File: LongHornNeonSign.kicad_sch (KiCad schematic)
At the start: 61 parts, among them J1 Screw_Terminal_01x02, J2 Screw_Terminal_01x02, J3 Screw_Terminal_01x02, J4 Screw_Terminal_01x02, Q1 AO3400A, Q2 AO3400A, Q3 AO3400A, Q4 AO3400A, SW1 SW_Push, SW2 SW_Push, SW3 SW_Push, U1 LM2596S-5

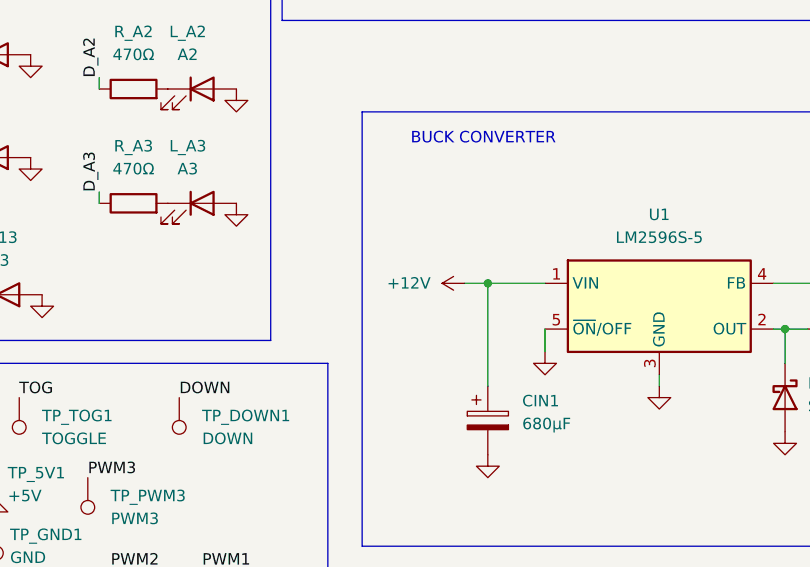
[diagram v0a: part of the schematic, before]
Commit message: May 12 2026 run it back
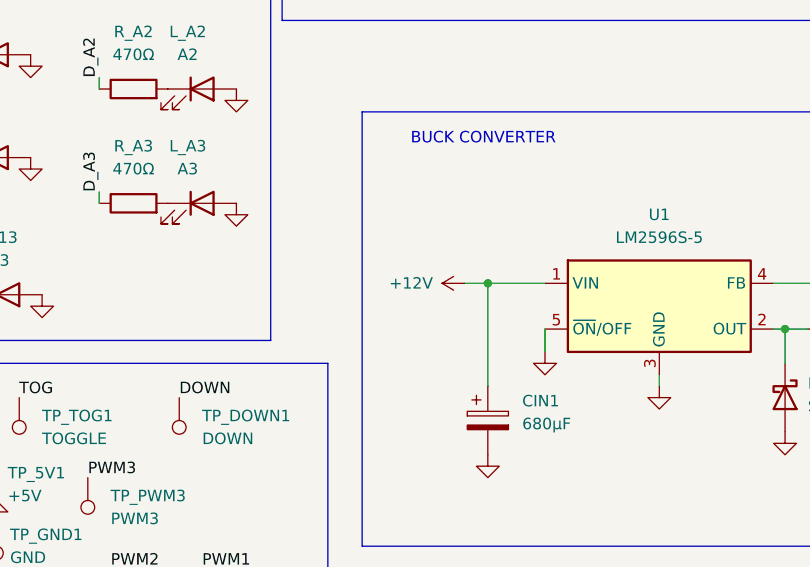
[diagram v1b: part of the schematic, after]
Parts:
- COUT1: footprint Capacitor_SMD:CP_Elec_8x10 -> Capacitor_SMD:CP_Elec_6.3x7.7; LCSC C976031 -> C2827940
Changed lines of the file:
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@@
 			)
 		)
-		(property "Footprint" "Capacitor_SMD:CP_Elec_8x10"
+		(property "Footprint" "Capacitor_SMD:CP_Elec_6.3x7.7"
 			(at 130.5052 118.11 0)
 			(effects
@@
 			)
 		)
-		(property "LCSC" "C976031"
+		(property "LCSC" "C2827940"
 			(at 129.54 114.3 0)
 			(effects
@@
 		(on_board yes)
 		(dnp no)
-		(fields_autoplaced yes)
 		(property "Reference" "#PWR031"
 			(at 85.09 101.6 0)
@@
 		)
 		(property "Value" "+12V"
-			(at 77.47 101.5999 90)
-			(effects
-				(font
+			(at 77.724 101.6 90)
+			(effects
+				(font
